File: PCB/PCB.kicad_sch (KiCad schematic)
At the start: 51 parts, among them J1 USB_C_Receptacle_USB2.0_16P, Q1 NMOS, SW1 RESET, SW2 Button, U1 RP2040, U2 W25Q32JVSS, U4 NCP1117-3.3_SOT223, Y1 12 MHz

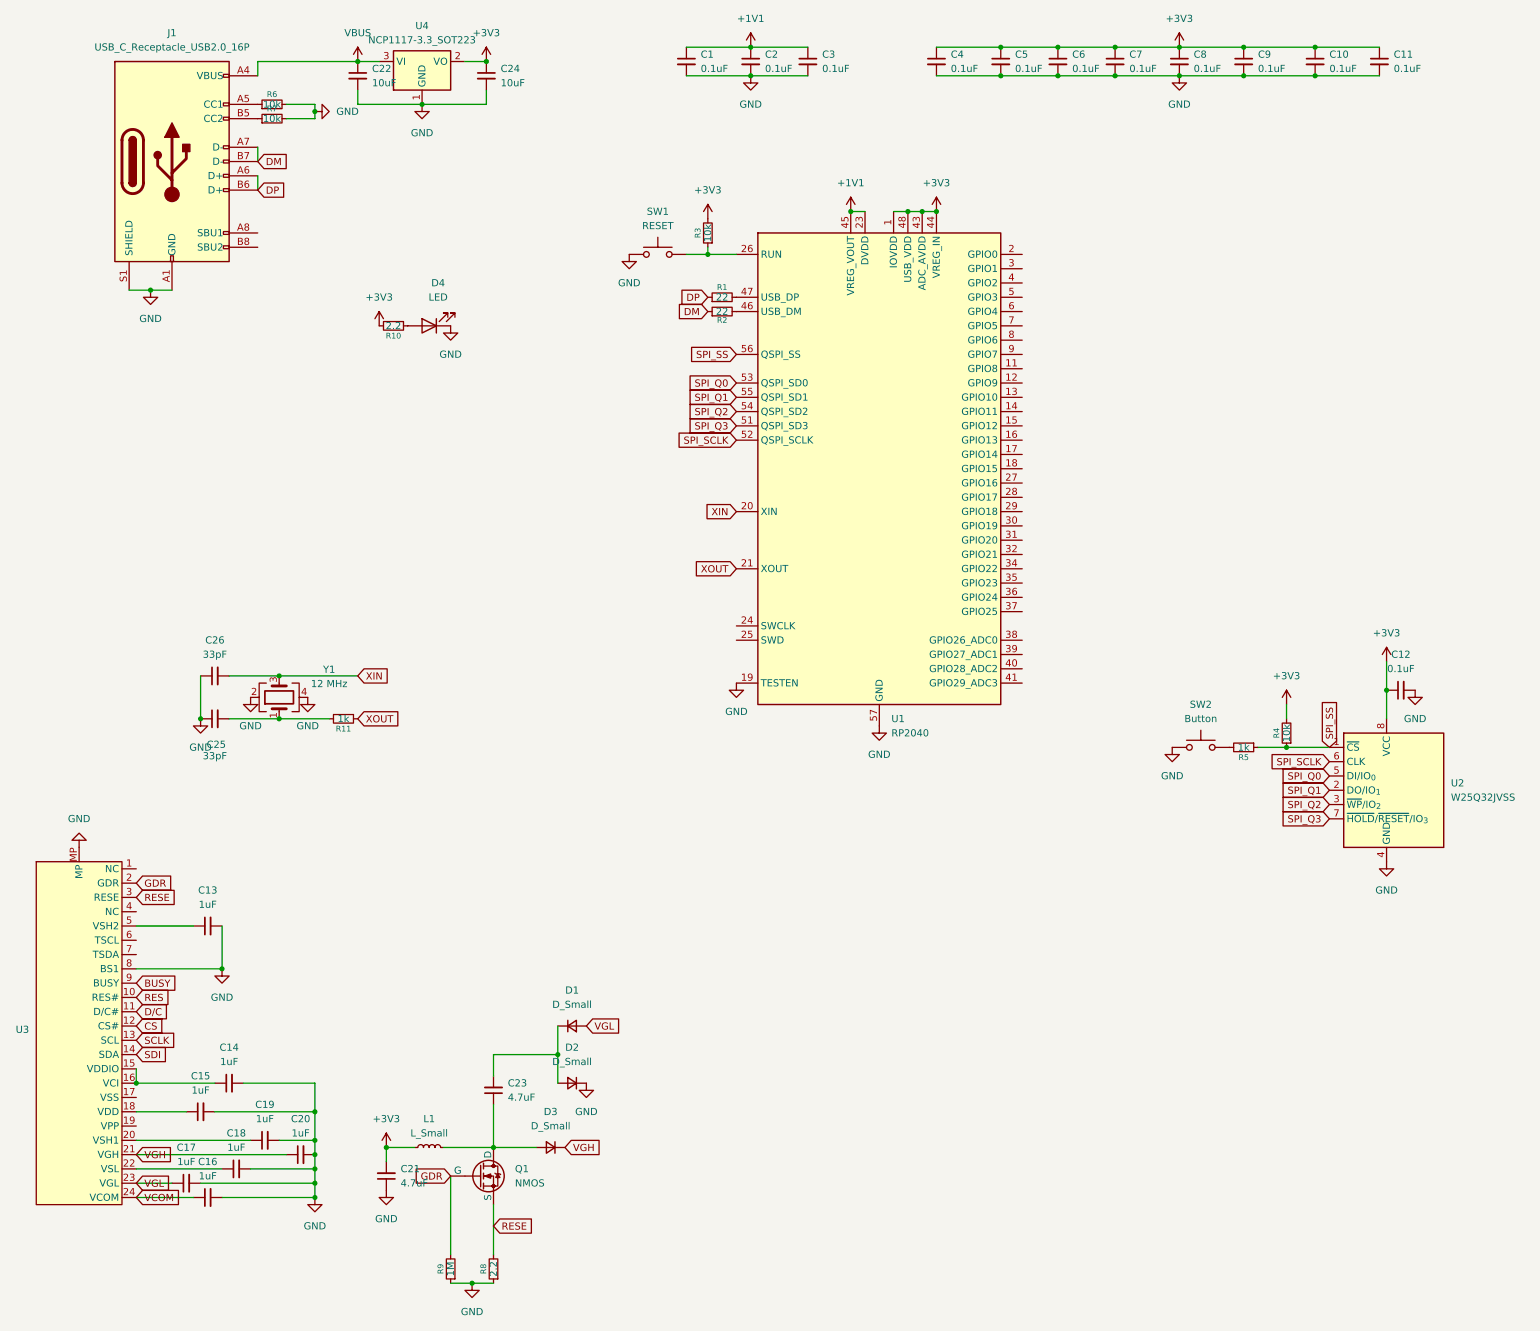
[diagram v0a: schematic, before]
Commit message: descriptive commit name
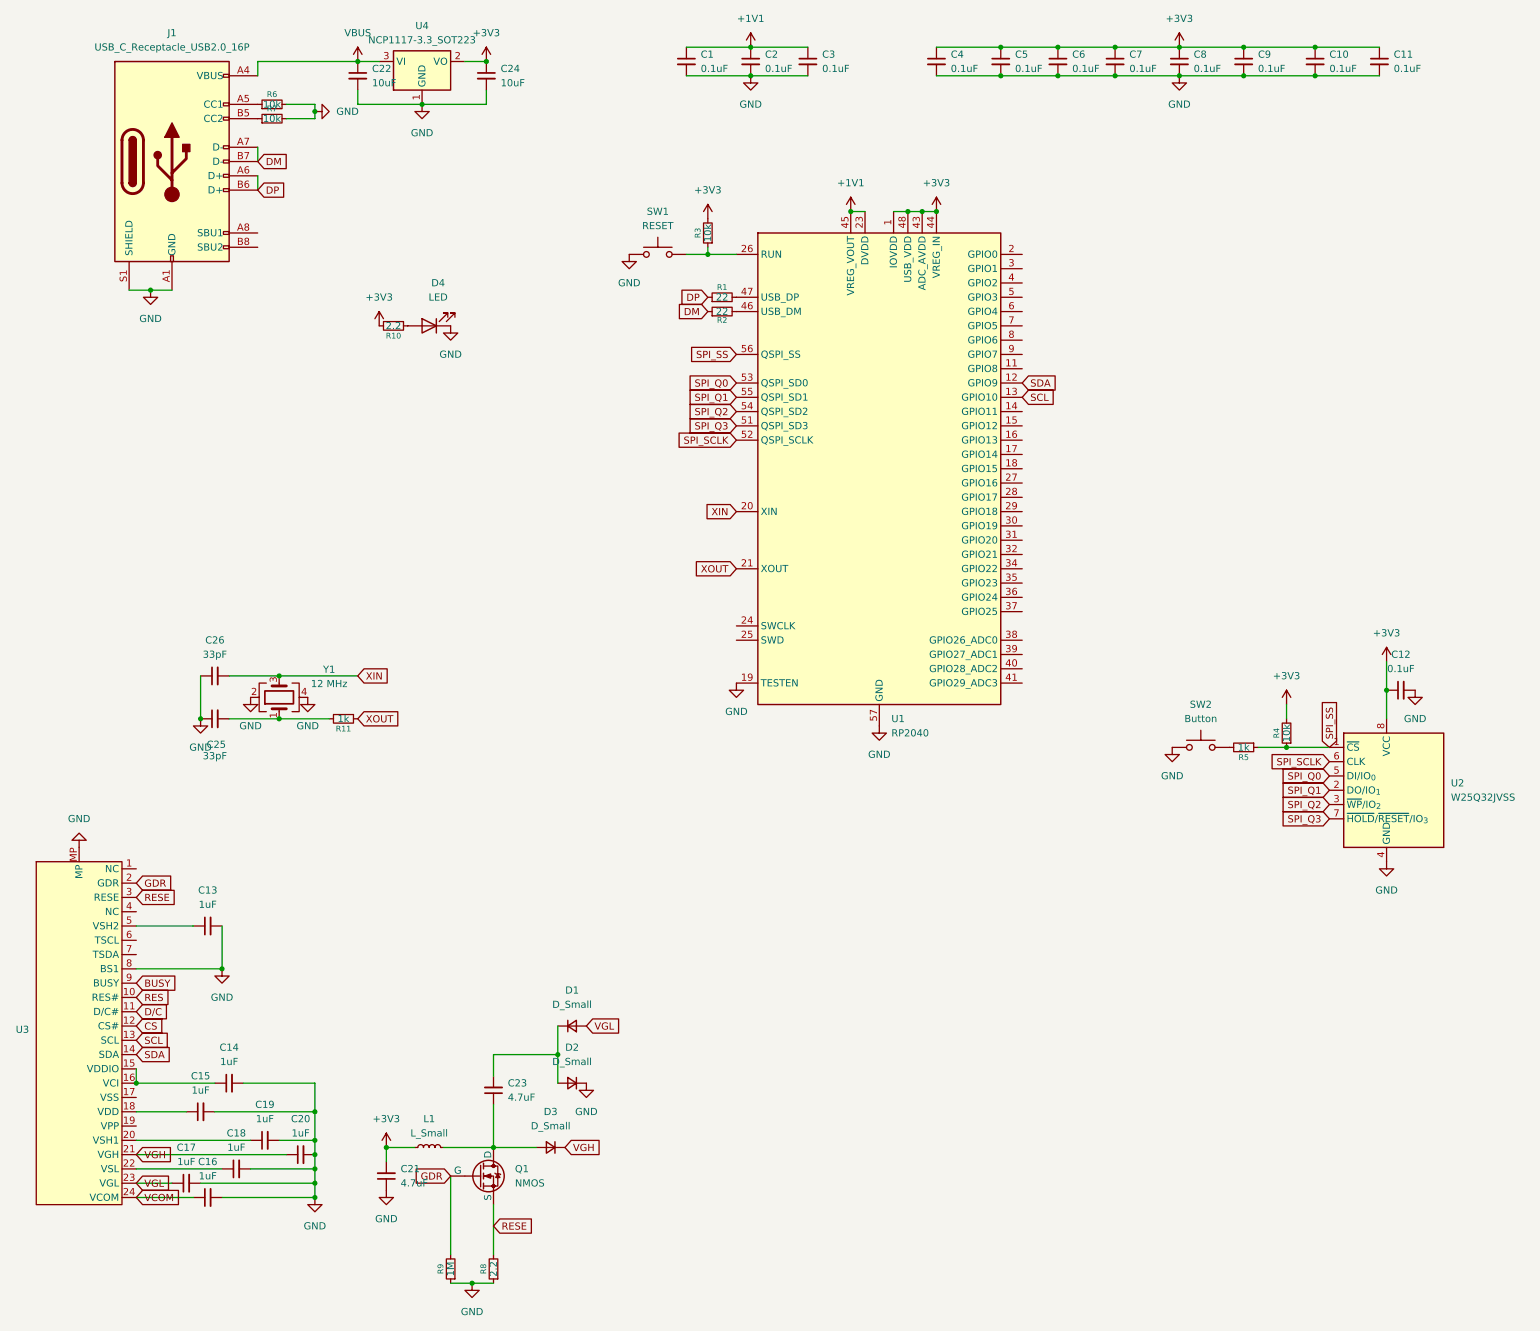
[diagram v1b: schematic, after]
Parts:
- Y1: footprint (none) -> Taranium-libs:CRYSTAL-SMD_4P-L3.2-W2.5-BL
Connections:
- net SCLK is gone; now on net SCL: U3.13 (SCL)
- net SDI is gone; now on net SDA: U3.14 (SDA)
- net SDA: now reaches U1.12 (GPIO9)
- net SCL: now reaches U1.13 (GPIO10)
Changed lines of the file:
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@@
 		)
 	)
+	(global_label "SDA"
+		(shape input)
+		(at 481.33 106.68 0)
+		(fields_autoplaced yes)
+		(effects
+			(font
+				(size 1.27 1.27)
+			)
+			(justify left)
+		)
+		(property "Intersheetrefs" "${INTERSHEET_REFS}"
+			(at 487.8833 106.68 0)
+			(effects
+				(font
+					(size 1.27 1.27)
+				)
+				(justify left)
+				(hide yes)
+			)
+		)
+	)
 	(global_label "SPI_Q0"
 		(shape input)
@@
 		)
 	)
-	(global_label "SCLK"
+	(global_label "SCL"
 		(shape input)
 		(at 323.85 223.52 0)
@@
 		)
 		(property "Intersheetrefs" "${INTERSHEET_REFS}"
-			(at 331.6128 223.52 0)
+			(at 330.3428 223.52 0)
 			(effects
 				(font
@@
 		)
 	)
-	(global_label "SDI"
+	(global_label "SDA"
 		(shape input)
 		(at 323.85 226.06 0)
@@
 		)
 		(property "Intersheetrefs" "${INTERSHEET_REFS}"
-			(at 329.9195 226.06 0)
+			(at 330.4033 226.06 0)
 			(effects
 				(font
@@
 		)
 	)
+	(global_label "SCL"
+		(shape input)
+		(at 481.33 109.22 0)
+		(fields_autoplaced yes)
+		(effects
+			(font
+				(size 1.27 1.27)
+			)
+			(justify left)
+		)
+		(property "Intersheetrefs" "${INTERSHEET_REFS}"
+			(at 487.8228 109.22 0)
+			(effects
+				(font
+					(size 1.27 1.27)
+				)
+				(justify left)
+				(hide yes)
+			)
+		)
+	)
 	(global_label "XIN"
 		(shape input)
@@
 			)
 		)
-		(property "Footprint" ""
+		(property "Footprint" "Taranium-libs:CRYSTAL-SMD_4P-L3.2-W2.5-BL"
 			(at 349.25 162.56 0)
 			(effects

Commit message: push
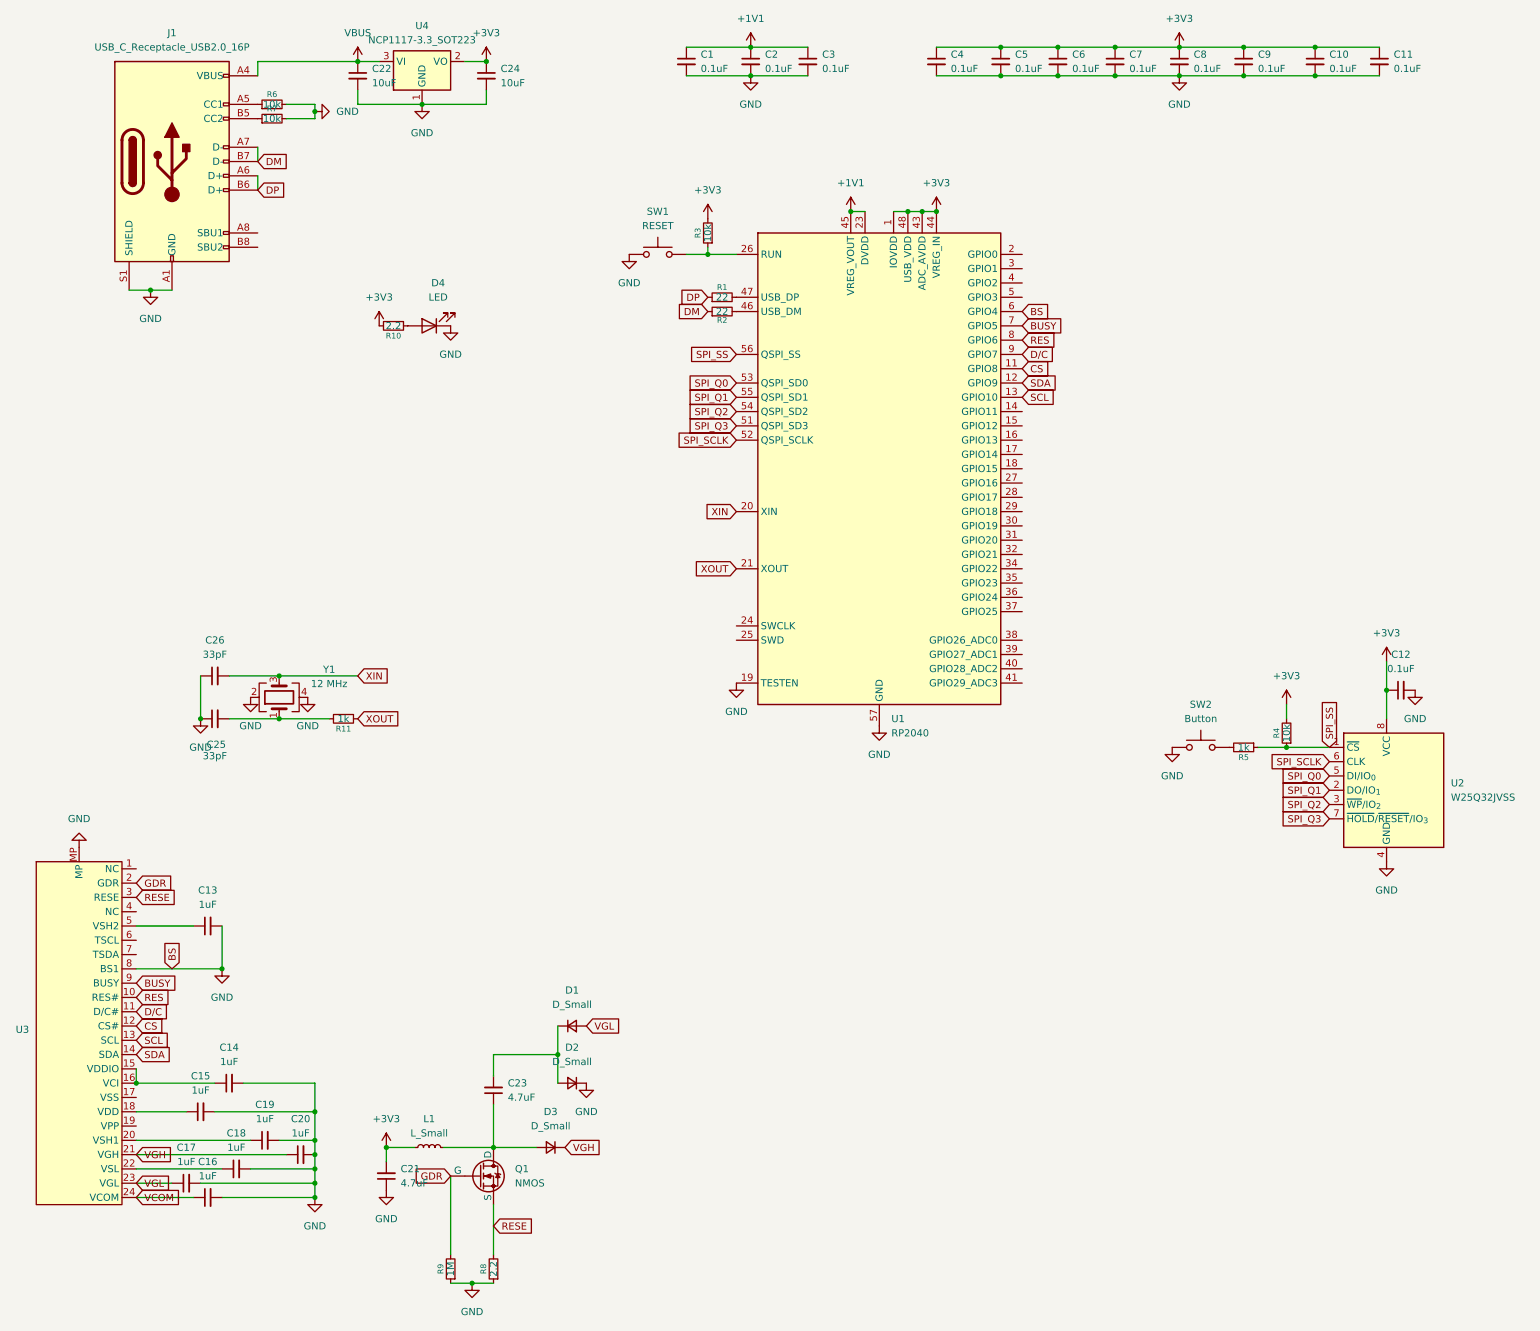
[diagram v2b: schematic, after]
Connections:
- net BUSY: now also U1.7 (GPIO5)
- net CS: now also U1.11 (GPIO8)
- net D/C: now also U1.9 (GPIO7)
- net GND: now also U1.6 (GPIO4)
- net RES: now also U1.8 (GPIO6)
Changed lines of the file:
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@@
+		)
+	)
+	(global_label "BUSY"
+		(shape input)
+		(at 481.33 96.52 0)
+		(fields_autoplaced yes)
+		(effects
+			(font
+				(size 1.27 1.27)
+			)
+			(justify left)
+		)
+		(property "Intersheetrefs" "${INTERSHEET_REFS}"
+			(at 489.2138 96.52 0)
+			(effects
+				(font
+					(size 1.27 1.27)
+				)
+				(justify left)
+				(hide yes)
+			)
 		)
 	)
@@
 		)
 	)
+	(global_label "RES"
+		(shape input)
+		(at 481.33 99.06 0)
+		(fields_autoplaced yes)
+		(effects
+			(font
+				(size 1.27 1.27)
+			)
+			(justify left)
+		)
+		(property "Intersheetrefs" "${INTERSHEET_REFS}"
+			(at 487.9437 99.06 0)
+			(effects
+				(font
+					(size 1.27 1.27)
+				)
+				(justify left)
+				(hide yes)
+			)
+		)
+	)
+	(global_label "BS"
+		(shape input)
+		(at 481.33 93.98 0)
+		(fields_autoplaced yes)
+		(effects
+			(font
+				(size 1.27 1.27)
+			)
+			(justify left)
+		)
+		(property "Intersheetrefs" "${INTERSHEET_REFS}"
+			(at 486.7947 93.98 0)
+			(effects
+				(font
+					(size 1.27 1.27)
+				)
+				(justify left)
+				(hide yes)
+			)
+		)
+	)
 	(global_label "DM"
 		(shape input)
@@
 		)
 	)
+	(global_label "CS"
+		(shape input)
+		(at 481.33 104.14 0)
+		(fields_autoplaced yes)
+		(effects
+			(font
+				(size 1.27 1.27)
+			)
+			(justify left)
+		)
+		(property "Intersheetrefs" "${INTERSHEET_REFS}"
+			(at 486.7947 104.14 0)
+			(effects
+				(font
+					(size 1.27 1.27)
+				)
+				(justify left)
+				(hide yes)
+			)
+		)
+	)
 	(global_label "DP"
 		(shape input)
@@
 		)
 	)
+	(global_label "BS"
+		(shape input)
+		(at 330.2 210.82 90)
+		(fields_autoplaced yes)
+		(effects
+			(font
+				(size 1.27 1.27)
+			)
+			(justify left)
+		)
+		(property "Intersheetrefs" "${INTERSHEET_REFS}"
+			(at 330.2 205.3553 90)
+			(effects
+				(font
+					(size 1.27 1.27)
+				)
+				(justify left)
+				(hide yes)
+			)
+		)
+	)
 	(global_label "XOUT"
 		(shape input)
@@
 				(hide yes)
 			)
+		)
+	)
+	(global_label "D{slash}C"
+		(shape input)
+		(at 481.33 101.6 0)
+		(fields_autoplaced yes)
+		(effects
+			(font
+				(size 1.27 1.27)
+			)
+			(justify left)
+		)
+		(property "Intersheetrefs" "${INTERSHEET_REFS}"
+			(at 488.1857 101.6 0)
+			(effects
+				(font
+					(size 1.27 1.27)
+				)
+				(justify left)
+				(hide yes)
+			)
